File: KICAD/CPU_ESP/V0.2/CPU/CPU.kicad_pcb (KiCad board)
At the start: 2 copper layers, 100 x 100 mm, 82 parts, among them J101 USB_B_Mini, J102 Conn_01x04, J501 Conn_02x20_Odd_Even, J502 Conn_02x20_Odd_Even, Q601 BSR19, Q602 BSR19, SW101 SW_Push_45deg, SW102 SW_Push_45deg, U201 LM75A, U202 PCA9306, U203 PCF8563T, U204 TCA9544A, U205 MCP23017_SS, U207 AT24CS01-SSHM, U301 LM1117DT-2.5, U401 ESP32-WROOM-32, U402 FT232RL, U403 TJA1051T, U601 SAA1064T, Y201 32.278kHz

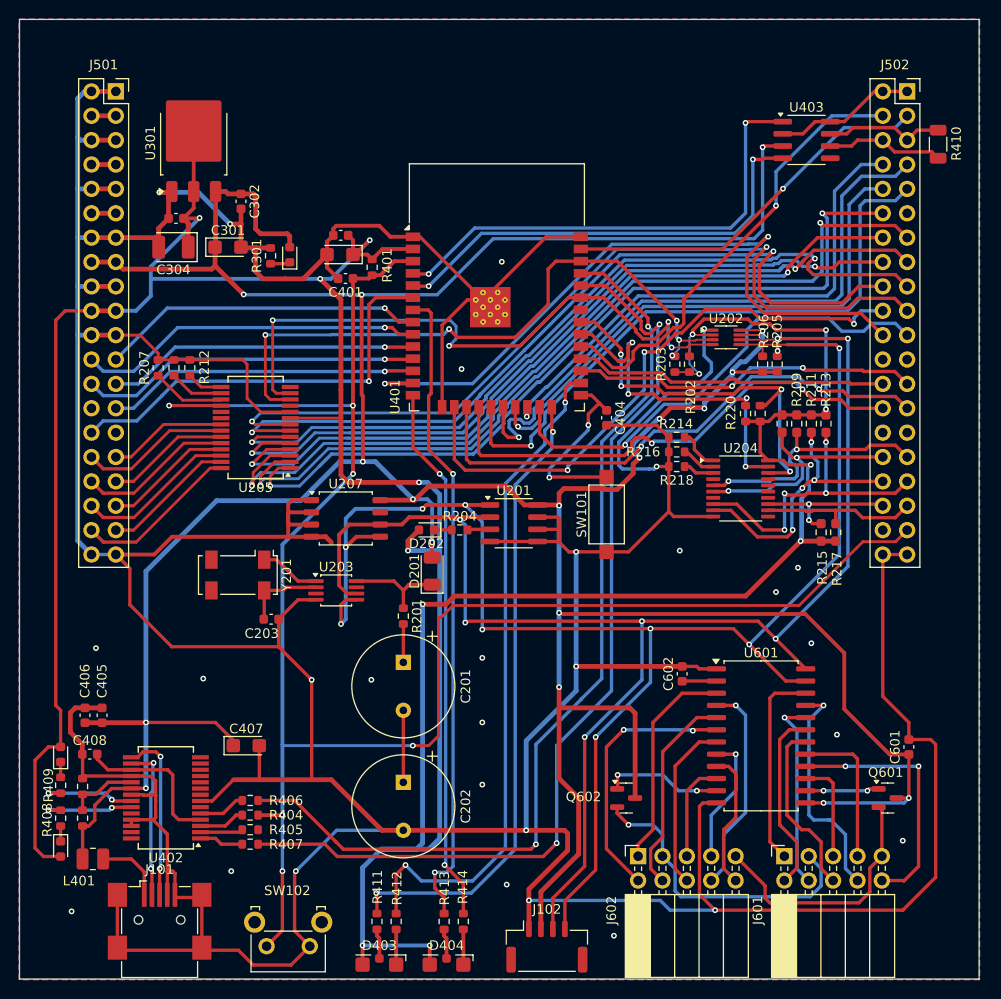
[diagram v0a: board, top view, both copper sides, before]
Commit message: KICAD CMOS  CPU V0.2
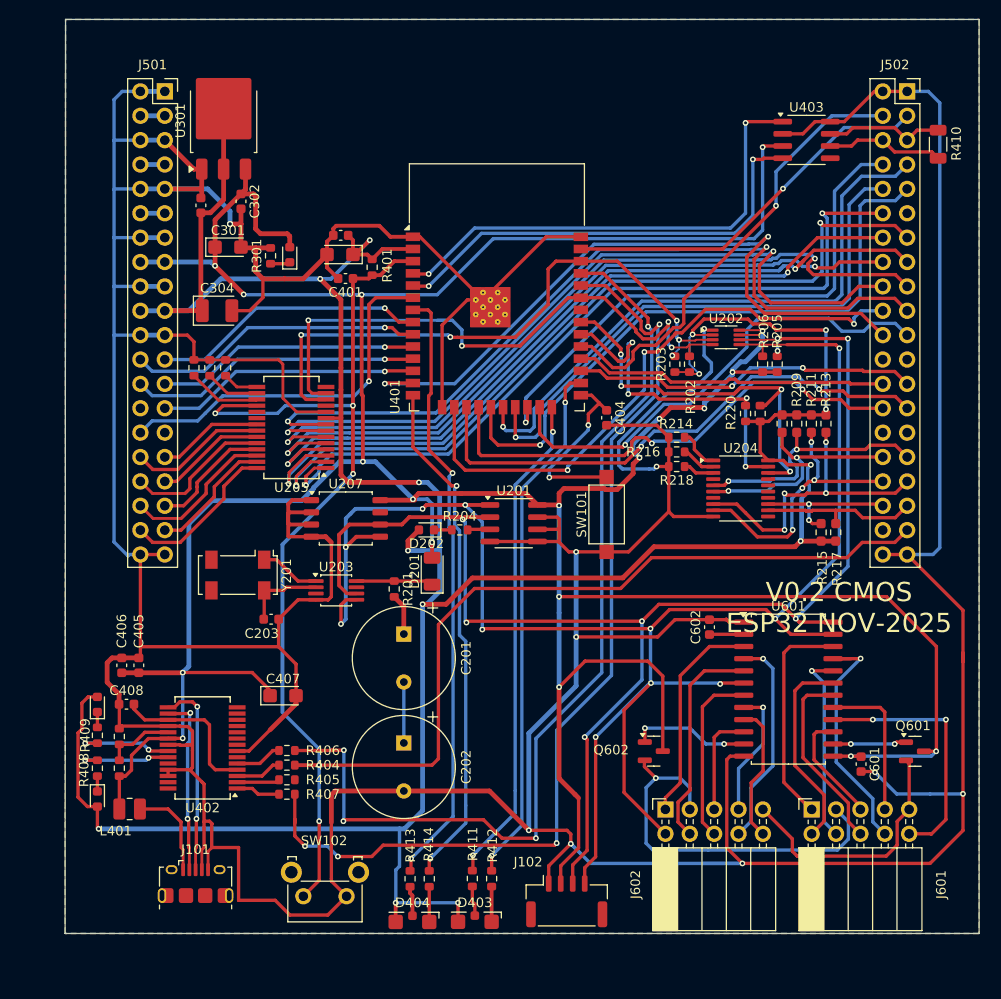
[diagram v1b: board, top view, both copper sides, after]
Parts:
- J101: value USB_B_Mini -> USB_B_Micro; footprint Connector_USB:USB_Mini-B_Wuerth_65100516121_Horizontal -> Connector_USB:USB_Micro-B_Amphenol_10118194-0001LF_Horizontal
- moved D403 10.9 mm to (172.4, 149.0)
- moved R412 10.9 mm to (174.2, 144.0)
- moved R411 10.9 mm to (172.2, 144.0)
- moved C304 8.03 mm to (145.6, 84.8), turned to 0 degrees
- moved D401 6.46 mm to (133.1, 135.7)
- moved C406 6.46 mm to (135.7, 121.8)
- moved C408 6.46 mm to (136.2, 125.9)
- moved C407 6.46 mm to (152.5, 125.0)
- moved R402 6.46 mm to (135.4, 129.2)
- moved D402 6.46 mm to (133.1, 125.9)
- moved L401 6.46 mm to (136.5, 136.8)
- moved R404 6.46 mm to (152.9, 132.2)
- moved R405 6.46 mm to (152.9, 133.7)
- moved R406 6.46 mm to (152.9, 130.7)
- moved R407 6.46 mm to (152.9, 135.2)
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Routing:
- net +3.3V: track 383.1 -> 319.3 mm
- net +5VD: track 430.1 -> 396.5 mm, vias 18 -> 19
- net GND: track 673.6 -> 689.1 mm, vias 29 -> 11
- net Net-(U401-IO4): track 70.3 -> 55.3 mm
- net Net-(U401-IO2): track 66.3 -> 51.8 mm
- net /RESET: track 189.1 -> 178.2 mm, vias 6 -> 5
- net Net-(J601-Pin_3): track 32.3 -> 41.2 mm
- net /SDA-5V: track 166.3 -> 159.4 mm
- net /SCL-5V: track 156.5 -> 150.3 mm
- net /D0: track 86.5 -> 80.7 mm
- net /PWM4: track 32.6 -> 27.5 mm
- net /PWM0: track 33.8 -> 28.7 mm
- net /PWM2: track 32.6 -> 27.5 mm
- net /PWM3: track 35.6 -> 30.5 mm
- net /IO8: track 44.0 -> 38.9 mm
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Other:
- board size 100 x 100 mm -> 95.2 x 95.2 mm
- board text added: "V0.1 -> V 0.2 Correction taille PCB Correction position J501 et j502 Reprise du routage suite remise en place des composants USB MINI to MICRO"
- board text added: "V0.2 CMOS ESP32 NOV-2025"
